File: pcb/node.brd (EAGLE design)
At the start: 25 x 25 mm, 12 parts, among them J1 AVR_SPI_PRG_62X3_LOCK

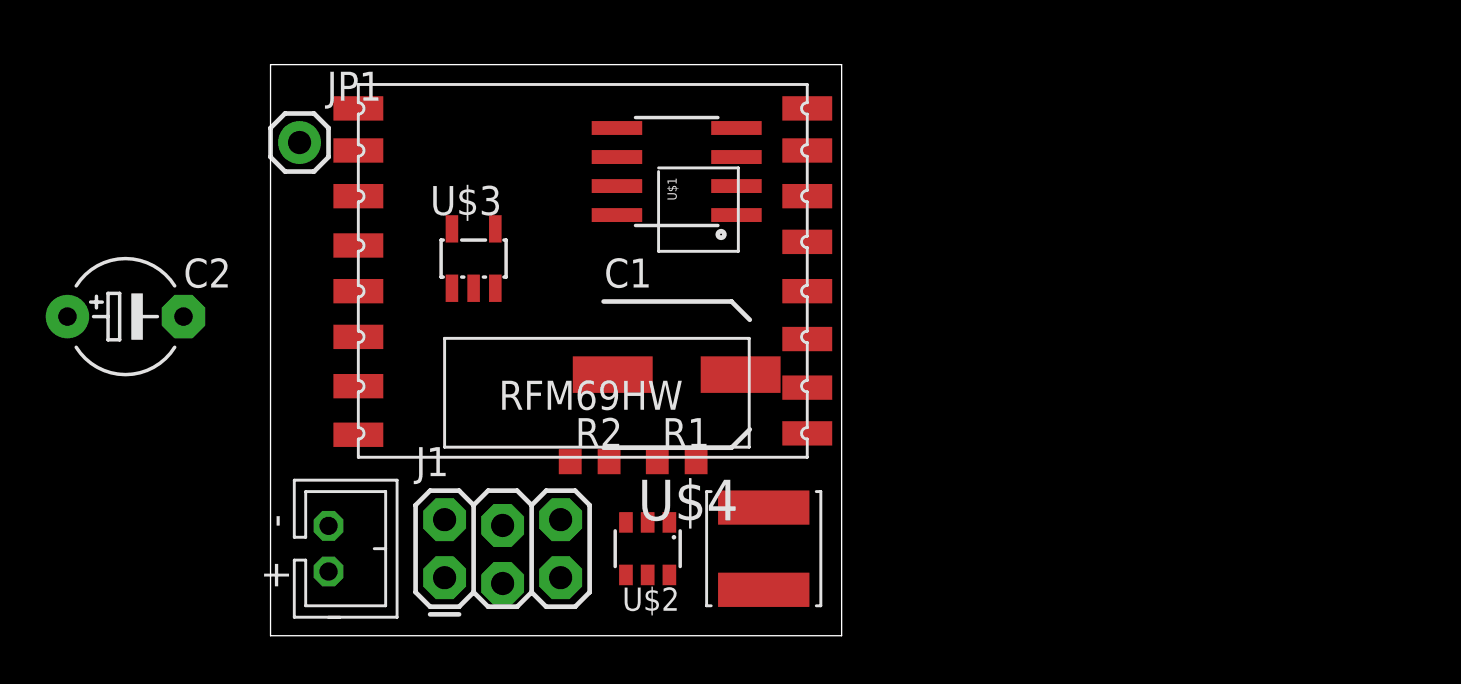
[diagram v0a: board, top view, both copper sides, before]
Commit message: routing commence
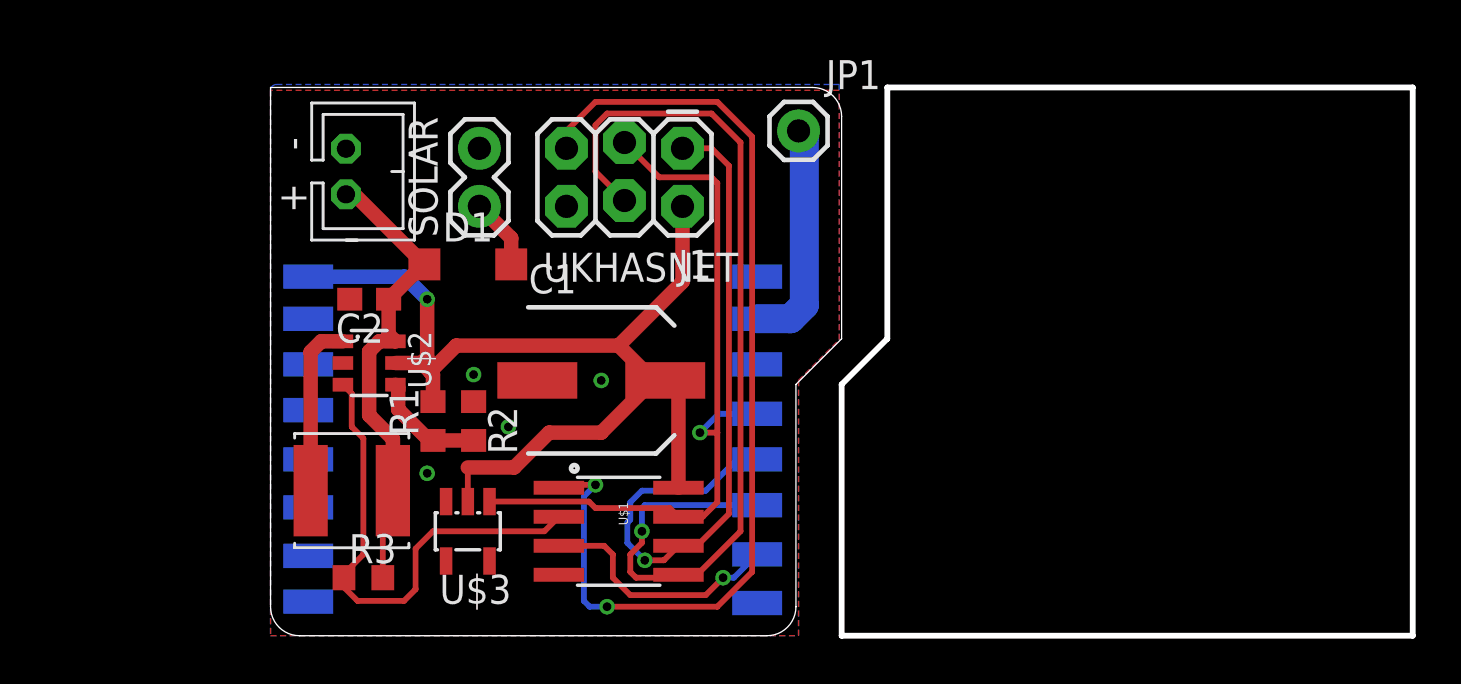
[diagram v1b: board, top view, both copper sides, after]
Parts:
- added D1: (no value), dtb:SOD123
- added R3: (no value), rcl:R0603
- added SOLAR: M02PTH, SparkFun-Connectors:1X02
- C2: device rcl:E5-5 -> rcl:C0603
- moved U$4 23.1 mm to (1.65, 16.8), flipped to the bottom
- moved JP1 21.8 mm to (23.1, 22.1)
- moved J1 21.5 mm to (18.0, 21.3), turned to 180 degrees
- moved DF 18.2 mm to (3.56, 6.35), turned to 180 degrees
- moved J2 16.5 mm to (3.30, 20.3)
- moved U$1 16.0 mm to (15.2, 4.57), turned to 270 degrees
- moved U$2 14.7 mm to (4.32, 11.9), turned to 270 degrees
- moved U$3 11.9 mm to (8.64, 4.57), turned to 180 degrees
- moved R1 10.8 mm to (7.11, 9.40), turned to 90 degrees
- moved C2 10.7 mm to (4.32, 14.7), turned to 180 degrees
- moved R2 5.38 mm to (8.89, 9.40), turned to 270 degrees
- moved C1 3.31 mm to (14.5, 11.2)
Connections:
- new net N$5: D1.A, SOLAR.1
- net GND: now also C2.2, SOLAR.2; no longer C2.-
- net N$4: now also R3.1
- net VBATT: now also C2.1, D1.C, R3.2; no longer C2.+
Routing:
- net VCC: track 0.00 -> 46.3 mm, vias 0 -> 1
- net RESET: track 0.00 -> 44.3 mm, vias 0 -> 2
- net MOSI: track 0.00 -> 42.0 mm, vias 0 -> 1
- net DET/SCK: track 0.00 -> 32.9 mm, vias 0 -> 1
- net MISO: track 0.00 -> 31.4 mm, vias 0 -> 1
- net VBATT: track 0.00 -> 22.2 mm
- net N$4: track 0.00 -> 21.9 mm
- net RFM_SS: track 0.00 -> 11.7 mm, vias 0 -> 1
- net N$3: track 0.00 -> 10.0 mm
- net N$1: track 0.00 -> 8.01 mm
- net N$2: track 0.00 -> 5.00 mm
- net N$5: track 0.00 -> 3.12 mm
- added copper zone on layer 1, net GND
- added copper zone on layer 16, net GND
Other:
- board size 25 x 25 mm -> 50 x 24 mm
- board text added: "UKHASNET"
